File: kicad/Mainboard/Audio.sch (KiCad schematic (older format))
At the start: 45 parts, among them J10 SPK_INT, J11 SPK_EXT, J8 MIC_INT, J9 MIC_EXT, SW1 INT_PTT_SW, U7 OPA340UA, U8 LM386

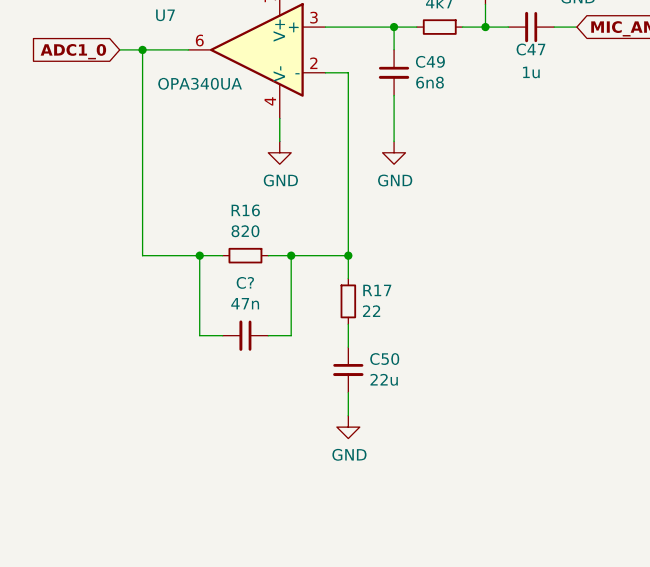
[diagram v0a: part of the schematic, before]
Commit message: Annotated parts
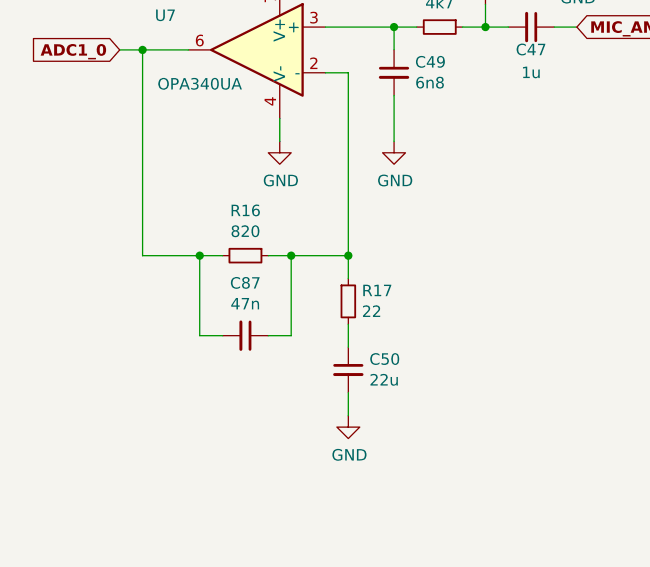
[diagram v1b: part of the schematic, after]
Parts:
- gave numbers to parts that had none: 1
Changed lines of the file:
@@
 	4200 5300 4200 5800
 $Comp
-L Device:C_Small C?
+L Device:C_Small C87
 U 1 1 5E069A61
 P 1450 2950
-F 0 "C?" V 1221 2950 50  0000 C CNN
+F 0 "C87" V 1221 2950 50  0000 C CNN
 F 1 "47n" V 1312 2950 50  0000 C CNN
 F 2 "" H 1450 2950 50  0001 C CNN
